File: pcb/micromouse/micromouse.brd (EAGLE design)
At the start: 80 x 115 mm, 70 parts, among them IC1 LM2575-5.0WU-(TR), IC2 LM2575-3.3WU-(TR), IC3 DSPIC33FJ64MC804-PT, IC4 L293D, Y1 7.3728MHz

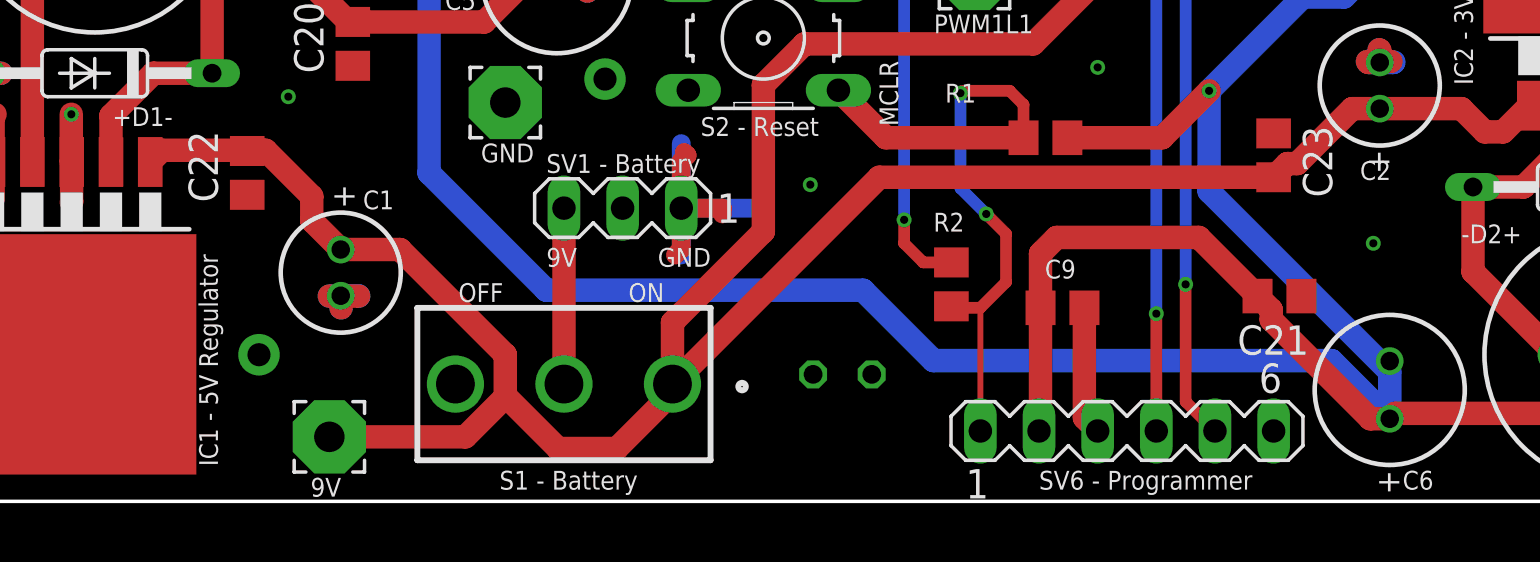
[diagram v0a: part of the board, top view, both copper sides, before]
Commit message: Fix minor issues from previous commit.
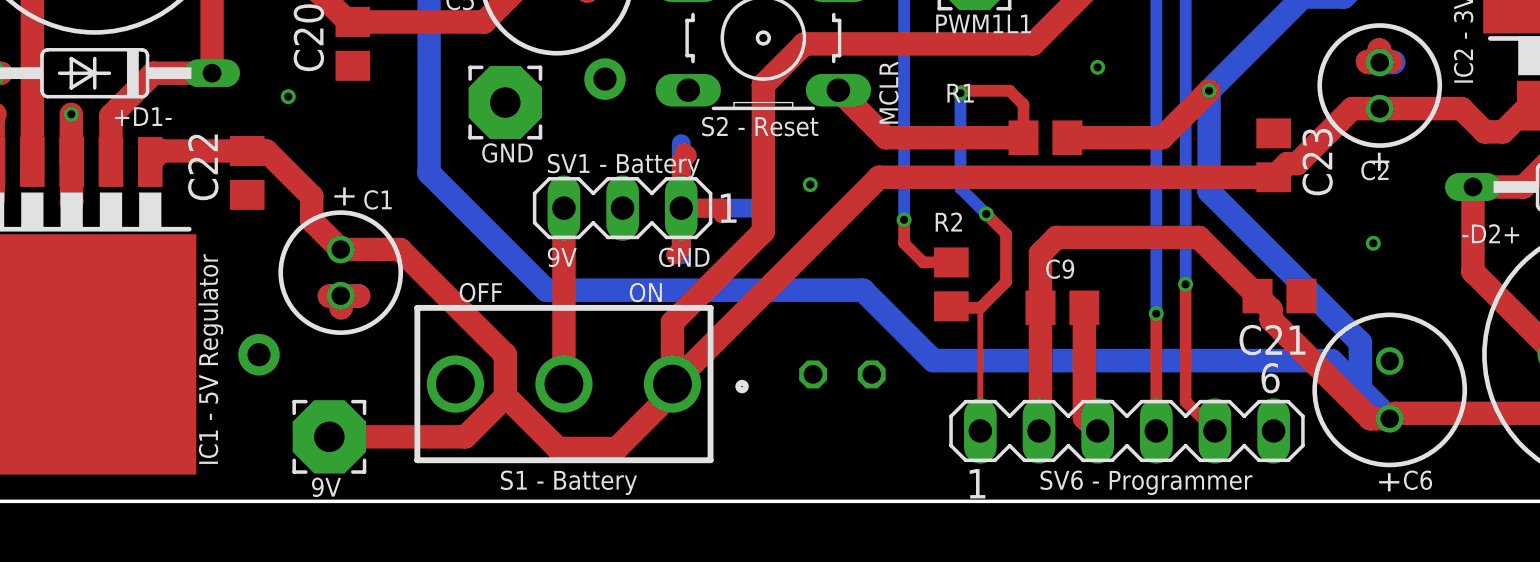
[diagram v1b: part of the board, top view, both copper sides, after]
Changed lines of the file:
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@@
 <drawing>
 <settings>
-<setting alwaysvectorfont="yes"/>
+<setting alwaysvectorfont="no"/>
 <setting verticaltext="up"/>
 </settings>
@@
 <wire x1="70.612" y1="37.592" x2="70.612" y2="36.3728" width="1.016" layer="1"/>
 <wire x1="55.88" y1="17.78" x2="55.88" y2="13.4312" width="1.016" layer="16"/>
-<wire x1="63.7032" y1="5.608" x2="63.7032" y2="3.576" width="1.016" layer="16"/>
-<wire x1="63.7032" y1="5.608" x2="55.88" y2="13.4312" width="1.016" layer="16"/>
+<wire x1="62.4332" y1="6.878" x2="62.4332" y2="4.846" width="1.016" layer="16"/>
+<wire x1="62.4332" y1="4.846" x2="63.7032" y2="3.576" width="1.016" layer="16"/>
+<wire x1="62.4332" y1="6.878" x2="55.88" y2="13.4312" width="1.016" layer="16"/>
 <wire x1="63.7032" y1="3.576" x2="61.1832" y2="6.096" width="1.016" layer="16"/>
 <wire x1="61.1832" y1="6.096" x2="43.942" y2="6.096" width="1.016" layer="16"/>
@@
 <wire x1="25.44785625" y1="4.52414375" x2="27.686" y2="2.286" width="1.016" layer="1"/>
 <wire x1="27.686" y1="2.286" x2="30.226" y2="2.286" width="1.016" layer="1"/>
-<wire x1="10.5316" y1="15.2052" x2="10.0236" y2="14.6972" width="1.016" layer="1"/>
 <wire x1="30.226" y1="2.286" x2="32.64" y2="4.7" width="1.016" layer="1"/>
 <wire x1="32.64" y1="4.7" x2="32.64" y2="5.08" width="1.016" layer="1"/>
@@
 <wire x1="20.844" y1="10.906" x2="18.272" y2="10.906" width="1.016" layer="1"/>
 <wire x1="18.272" y1="10.906" x2="17.018" y2="12.16" width="1.016" layer="1"/>
-<wire x1="17.018" y1="12.16" x2="17.018" y2="13.208" width="1.016" layer="1"/>
-<wire x1="17.018" y1="13.208" x2="15.0208" y2="15.2052" width="1.016" layer="1"/>
-<wire x1="15.0208" y1="15.2052" x2="10.5316" y2="15.2052" width="1.016" layer="1"/>
+<wire x1="17.018" y1="13.208" x2="17.018" y2="12.16" width="1.016" layer="1"/>
 <wire x1="41.596" y1="14.036" x2="58.674" y2="14.036" width="1.016" layer="1"/>
 <wire x1="32.64" y1="5.08" x2="41.596" y2="14.036" width="1.016" layer="1"/>
@@
 <wire x1="62.07715" y1="17.0086" x2="63.2714" y2="17.0086" width="1.016" layer="1"/>
 <wire x1="59.69655" y1="14.628" x2="62.07715" y2="17.0086" width="1.016" layer="1"/>
-<wire x1="10.0236" y1="14.6972" x2="14.224" y2="15.174" width="0" layer="19" extent="1-1"/>
+<wire x1="14.224" y1="15.174" x2="15.052" y2="15.174" width="1.016" layer="1"/>
+<wire x1="15.052" y1="15.174" x2="17.018" y2="13.208" width="1.016" layer="1"/>
+<wire x1="10.0236" y1="14.6972" x2="10.5004" y2="15.174" width="1.016" layer="1"/>
+<wire x1="10.5004" y1="15.174" x2="14.224" y2="15.174" width="1.016" layer="1"/>
 </signal>
 <signal name="N$4">
